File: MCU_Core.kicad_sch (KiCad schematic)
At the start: 20 parts, among them U1 STM32F405RGTx

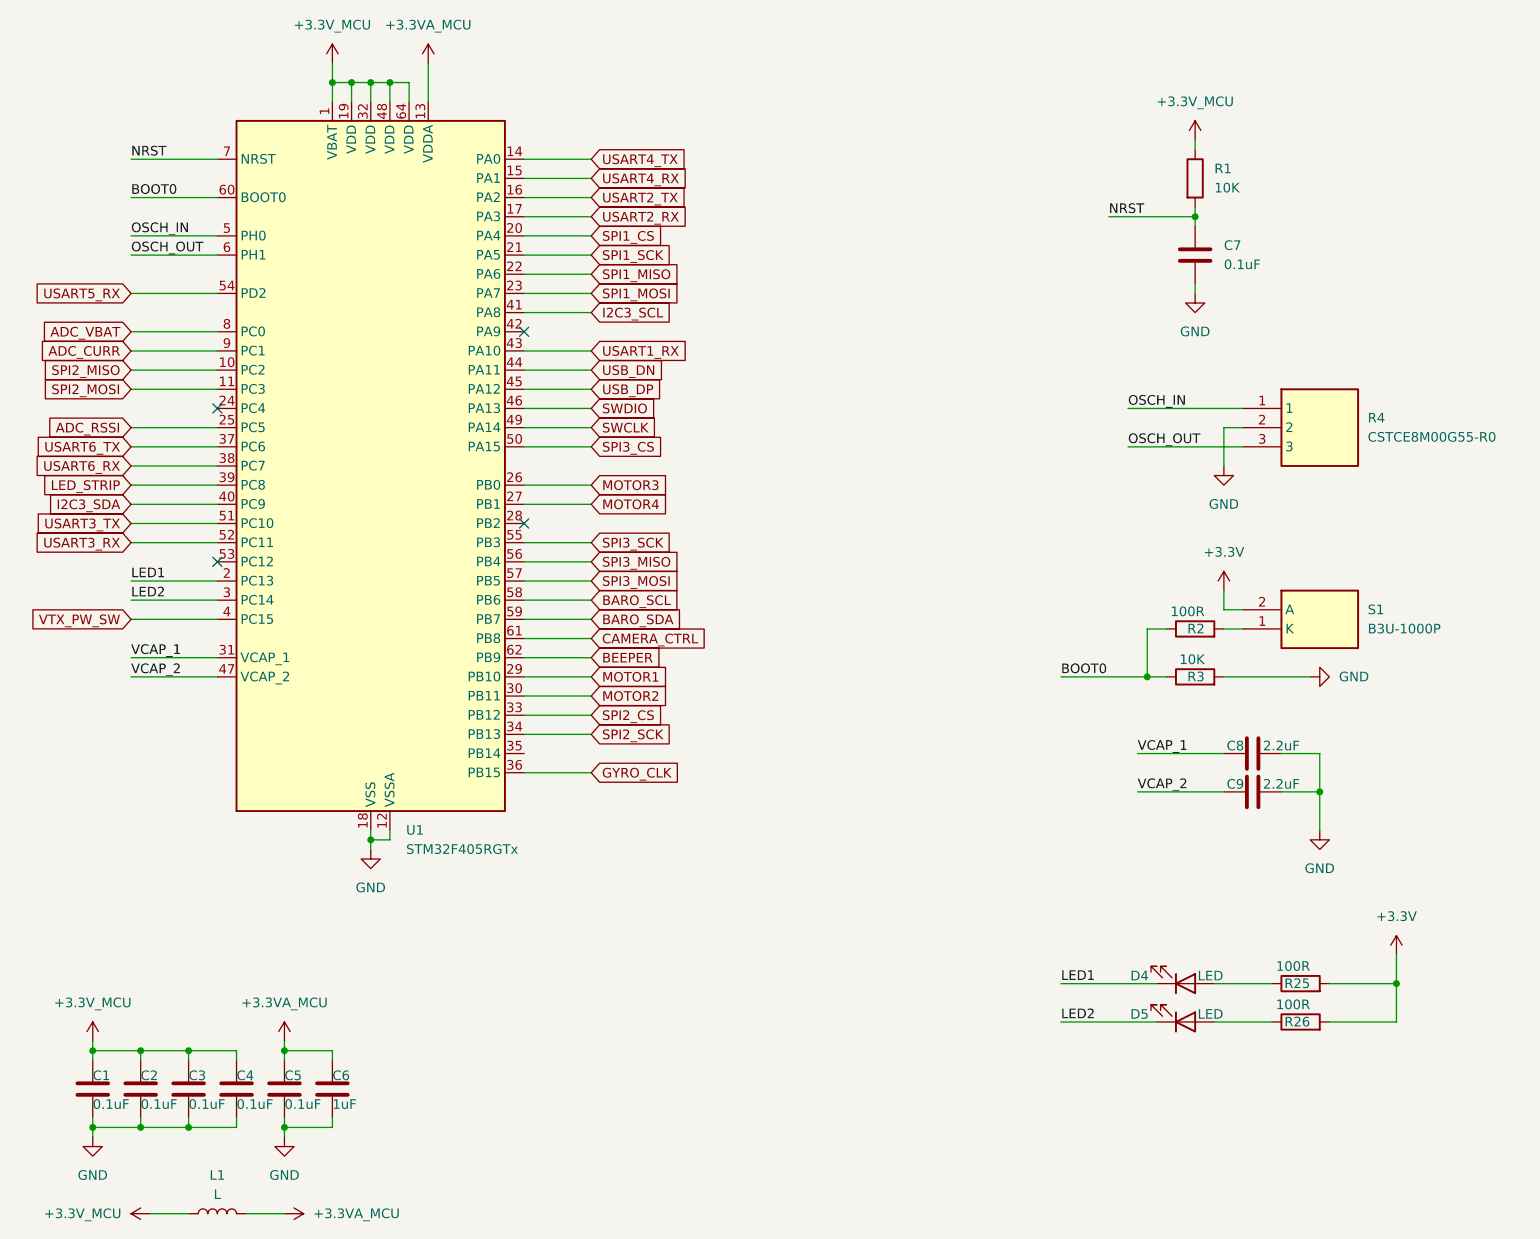
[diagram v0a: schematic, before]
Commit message: Update PCB Layout
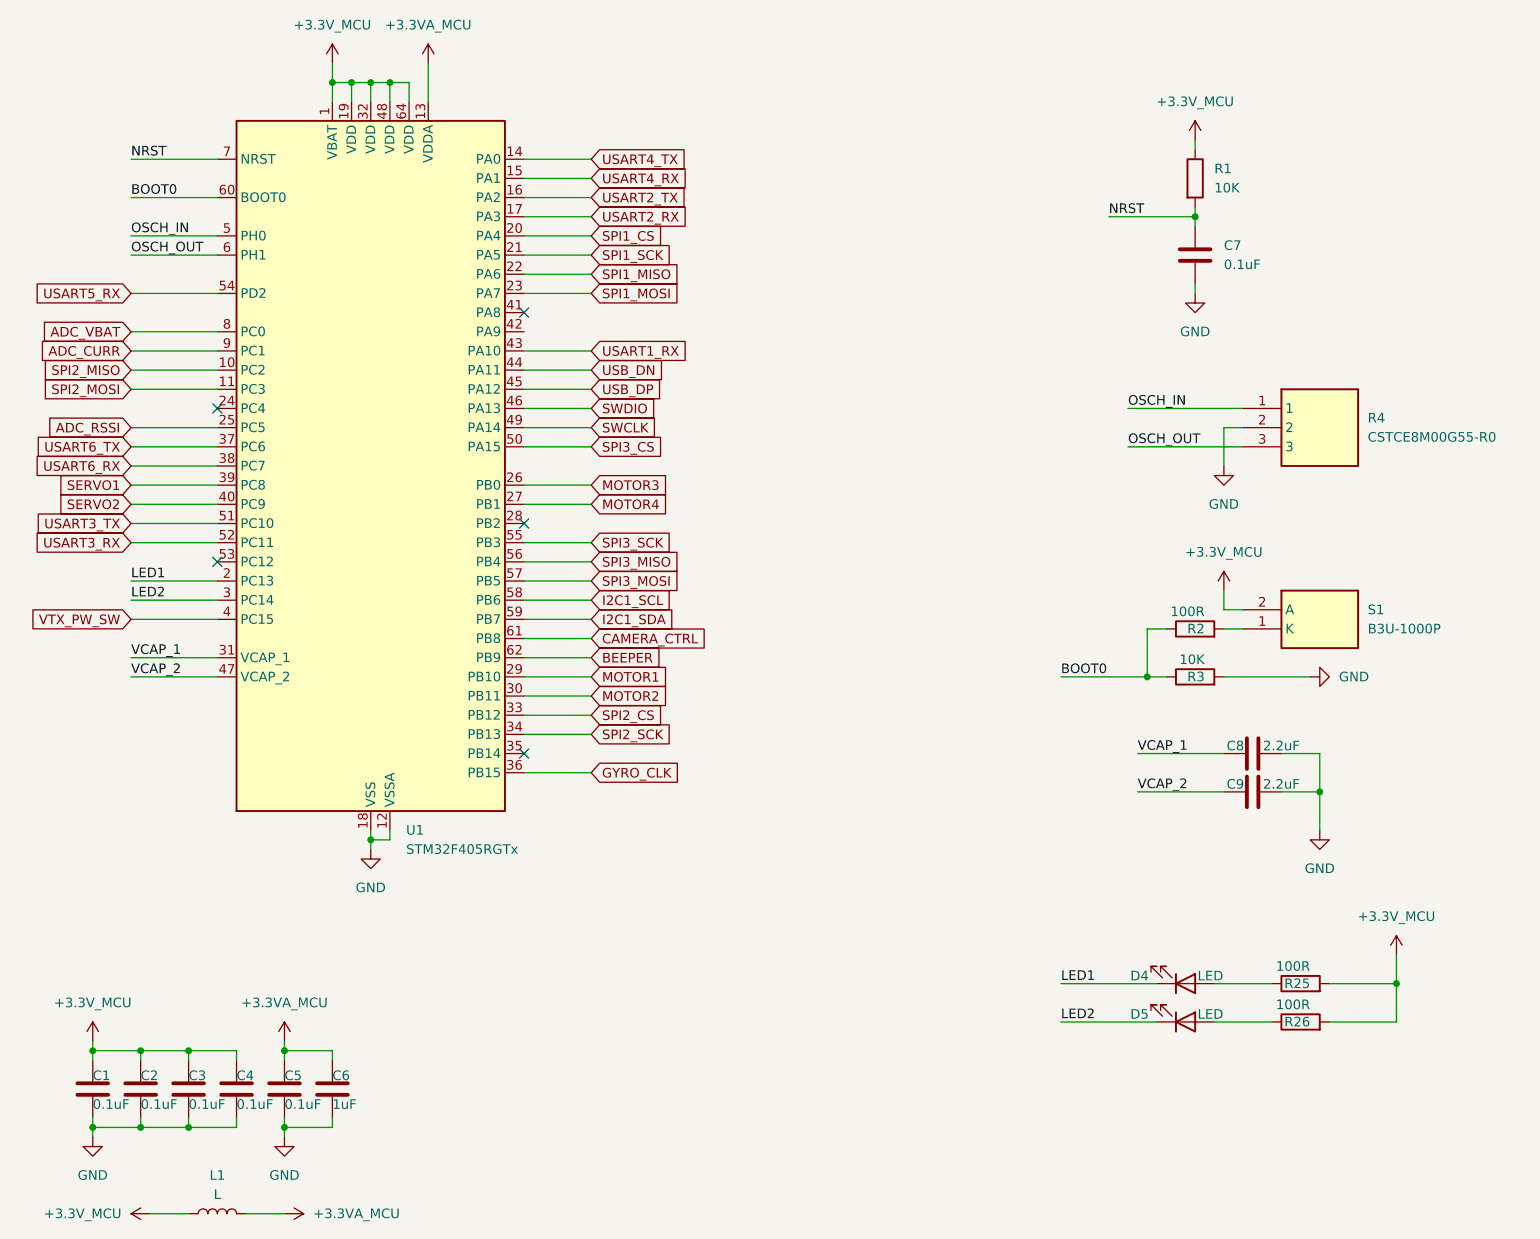
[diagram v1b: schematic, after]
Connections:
- net +3.3V is gone; now on net +3.3V_MCU: R25.2, R26.2, S1.2 (A)
- net BARO_SCL renamed I2C1_SCL
- net BARO_SDA renamed I2C1_SDA
- net I2C3_SCL: no longer names the net of U1.41 (PA8)
- net I2C3_SDA renamed SERVO2
- net LED_STRIP renamed SERVO1
- no-connect marks 4 -> 5
